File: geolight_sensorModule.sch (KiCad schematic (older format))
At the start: 18 parts, among them IC1 ATTINY841-SSU, P1 5V inject, P2 OPEN, P3 IN, P4 OUT, P5 AUX Sensor, P6 DEBUG, U1 TCRT5000/L, Y1 16Mhz

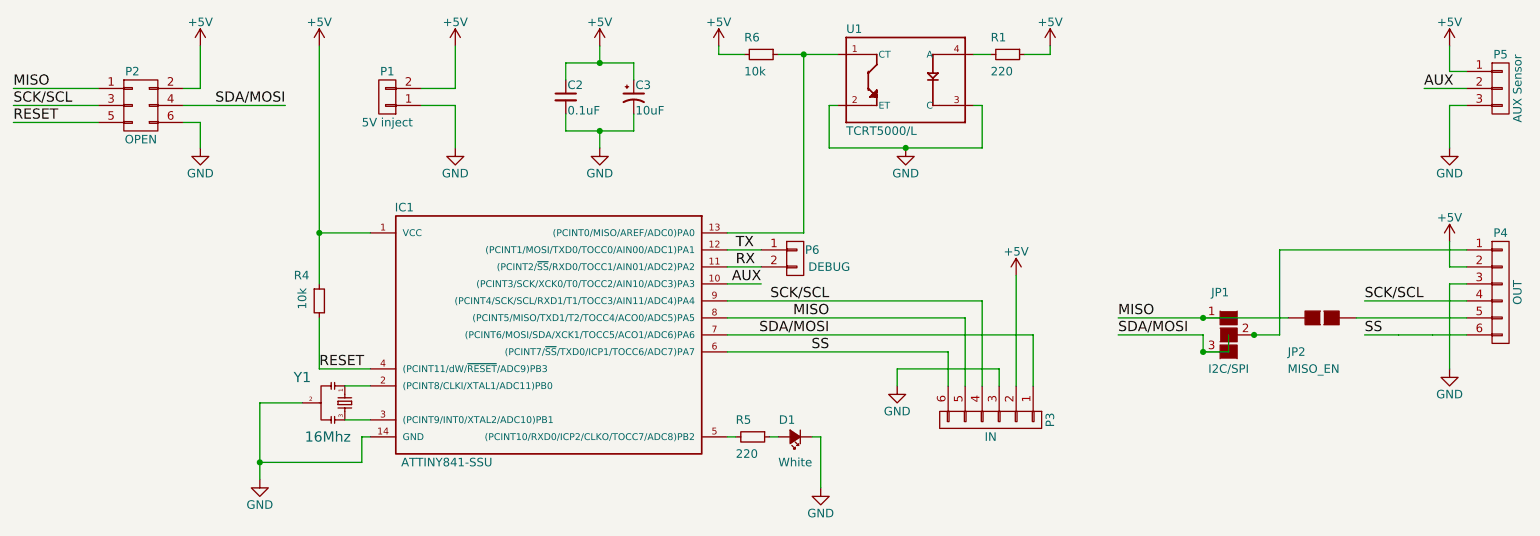
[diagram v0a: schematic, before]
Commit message: 5mm, rev2 stage (wait a day and finalize)
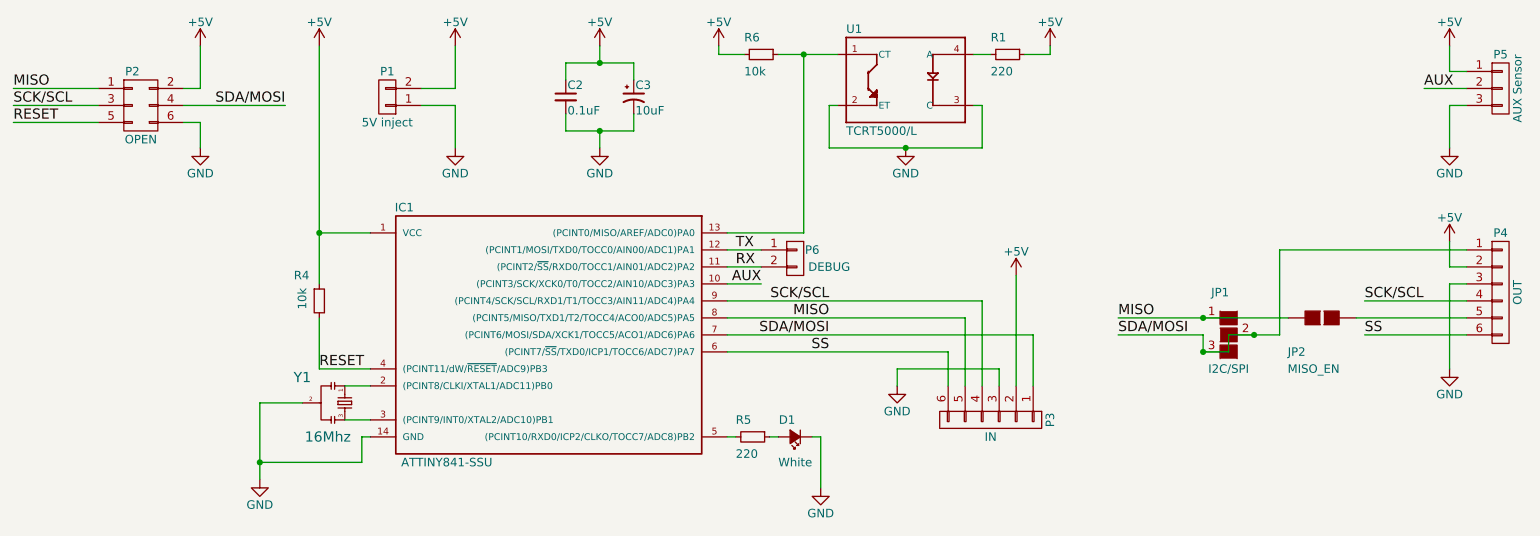
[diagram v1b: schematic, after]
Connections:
- net SDA/MOSI: now also JP1.2 (G2), P4.1 (P1)
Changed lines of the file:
@@
 	7550 4000 8050 4000
 Wire Wire Line
-	7550 3900 8050 3900
-Wire Wire Line
-	8050 3900 8550 3900
+	7550 3900 8550 3900
 Wire Wire Line
 	8200 4100 8200 4000
@@
 	8050 4100 8200 4100
 Wire Wire Line
-	9200 4000 9000 4000
+	9000 4000 9600 4000
 Wire Wire Line
-	5850 2900 6300 2900
-Wire Wire Line
-	6300 2900 6750 2900
+	5850 2900 6750 2900
 Wire Wire Line
 	4300 2700 4300 2800
@@
 	5900 2650 5850 2650
 Wire Wire Line
-	2500 4400 2500 4750
-Wire Wire Line
-	2500 4750 2500 4850
+	2500 4400 2500 4850
 Wire Wire Line
 	2750 4400 2500 4400
@@
 	2850 4200 2850 3900
 Wire Wire Line
-	2850 2300 2850 3400
-Wire Wire Line
-	2850 3400 2850 3700
+	2850 2300 2850 3700
 Wire Wire Line
 	4700 2800 4700 2700
@@
 	4700 2400 4700 2500
 Wire Wire Line
-	4300 2800 4500 2800
-Wire Wire Line
-	4500 2800 4700 2800
+	4300 2800 4700 2800
 Wire Wire Line
 	4500 2900 4500 2800
 Wire Wire Line
-	4300 2400 4500 2400
-Wire Wire Line
-	4500 2400 4700 2400
+	4300 2400 4700 2400
 Wire Wire Line
 	4500 2300 4500 2400
@@
 	5250 3600 5450 3600
 Wire Wire Line
-	5550 2350 5700 2350
-Wire Wire Line
-	5700 2350 5900 2350
+	5550 2350 5900 2350
 Wire Wire Line
 	5200 2300 5200 2350
@@
 	8950 3900 9600 3900
 Wire Wire Line
-	8350 4000 8500 4000
-Wire Wire Line
-	9200 4000 9400 4000
-Wire Wire Line
-	9400 4000 9600 4000
+	8200 4000 8500 4000
 Wire Wire Line
 	9500 3450 9500 3600
